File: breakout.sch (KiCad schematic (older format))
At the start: 24 parts, among them J1 JACK_TRS_4PINS, P1 CONN_01X08, P2 SPEAKER, P3 ISO7816_SIMPLE, P4 CONN_01X09, P5 SMA_CONN, P6 CONN_01X02, P7 USB_A, Q1 Q_PMOS_GSD, Q2 Q_NMOS_GSD, U1 SPX3819, U2 ESP-12E

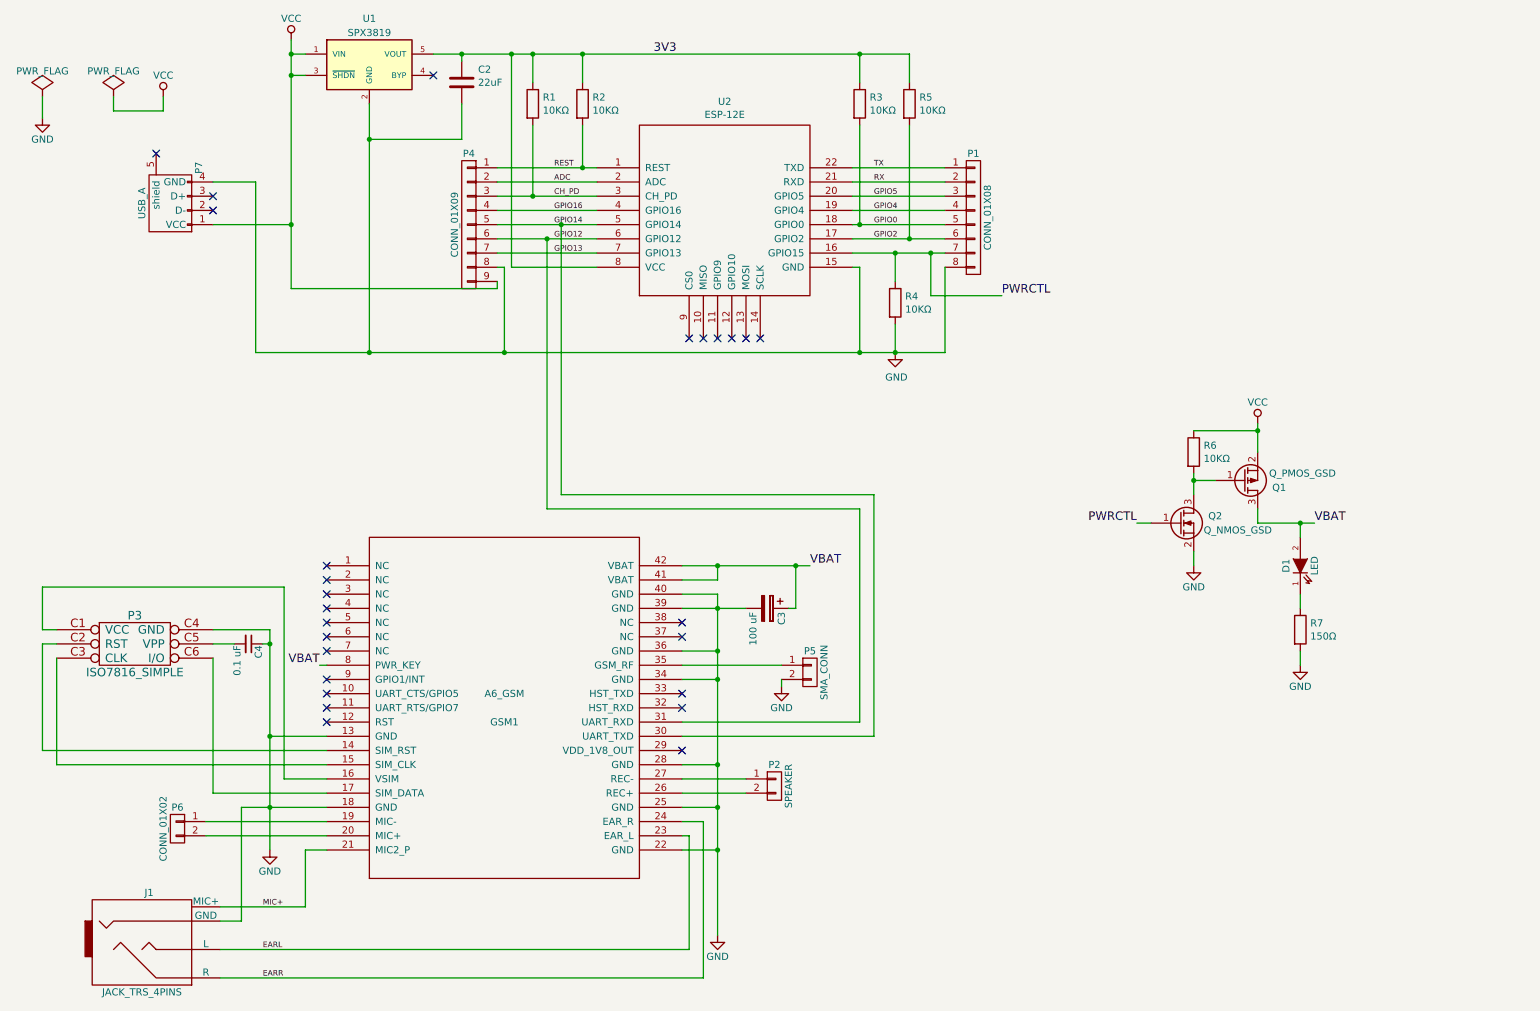
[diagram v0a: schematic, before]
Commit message: Add a bunch of audio crap.
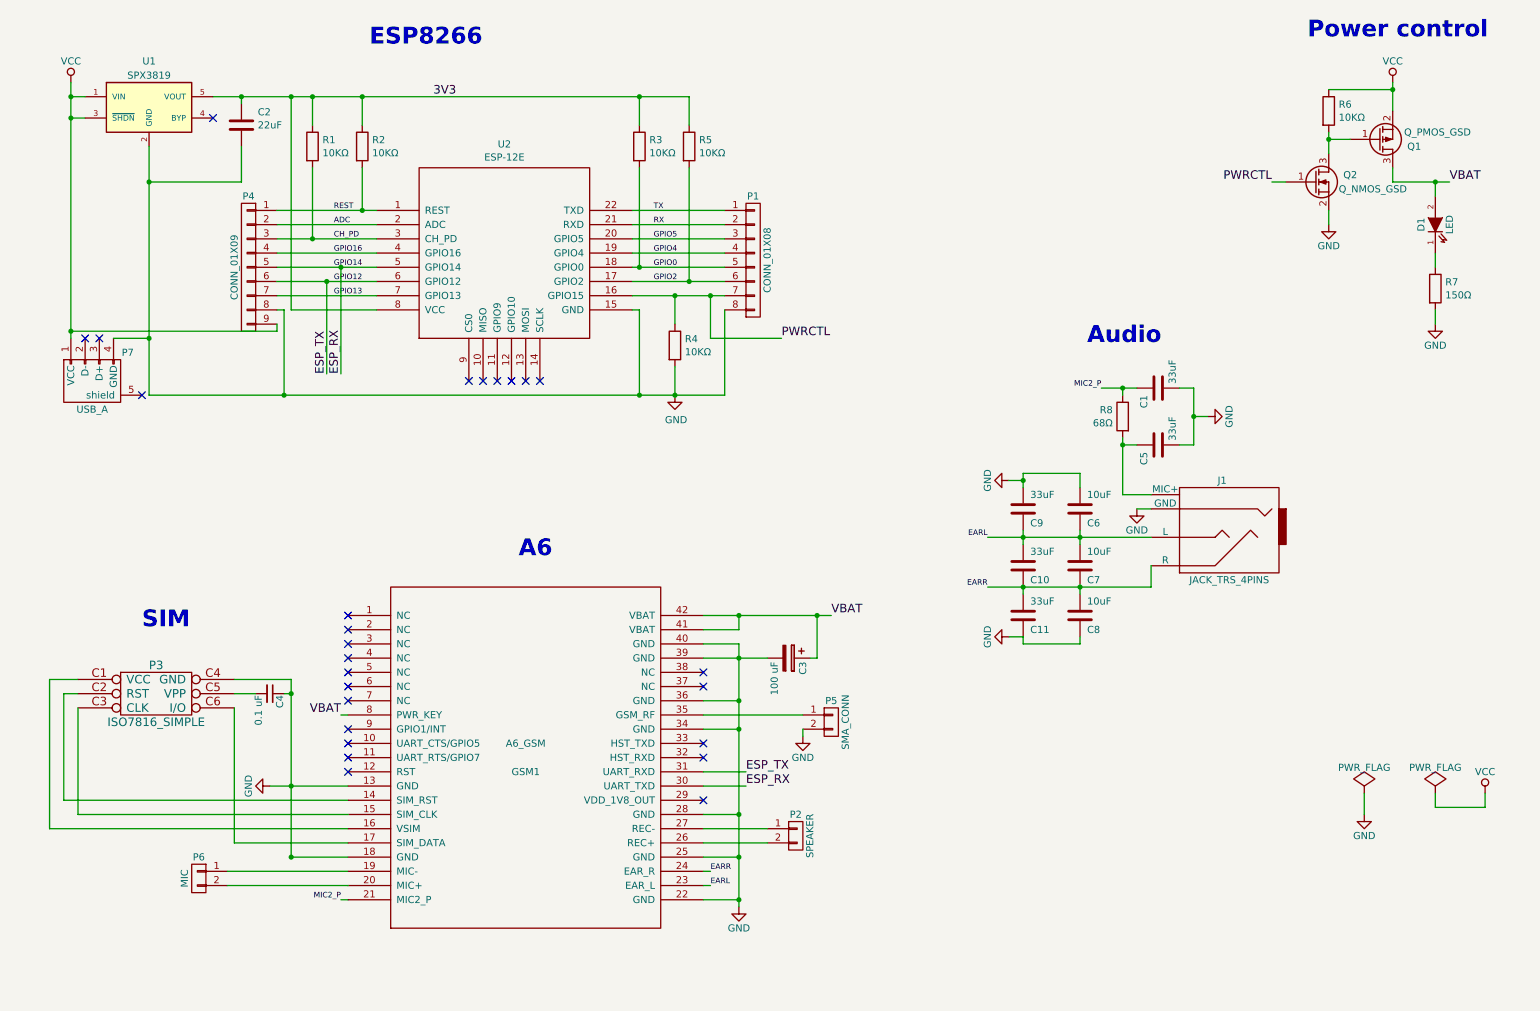
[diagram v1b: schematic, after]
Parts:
- added C1, C10, C11, C5, C9: 33uF, Capacitors_SMD:C_0805_HandSoldering, symbol C
- added C6, C7, C8: 10uF, Capacitors_SMD:C_0805_HandSoldering, symbol C
- added R8: 68Ω, Resistors_SMD:R_0805_HandSoldering, symbol R
- P6: value CONN_01X02 -> MIC
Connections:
- net EARL: now also C10.2, C6.1, C7.2, C9.1
- net EARR: now also C10.1, C11.2, C7.1, C8.2
- net GND: now also C1.2, C11.1, C5.2, C6.2, C8.1, C9.2
- net GPIO12 renamed ESP_TX
- net GPIO14 renamed ESP_RX
- net MIC+: no longer names the net of J1.5 (MIC+)
- net MIC+: now also C5.1, R8.2; no longer GSM1.21 (MIC2_P)
- new net MIC2_P: C1.1, GSM1.21 (MIC2_P), R8.1
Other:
- note added: "A6"
- note added: "Audio"
- note added: "ESP8266"
- note added: "Power control"
- note added: "SIM"
- moved on the sheet: C2, C3, C4, D1, GSM1, J1, P1, P2, P3, P4, P5, P6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
